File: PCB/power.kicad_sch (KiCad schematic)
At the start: 1 part, among them U2 LTC3370

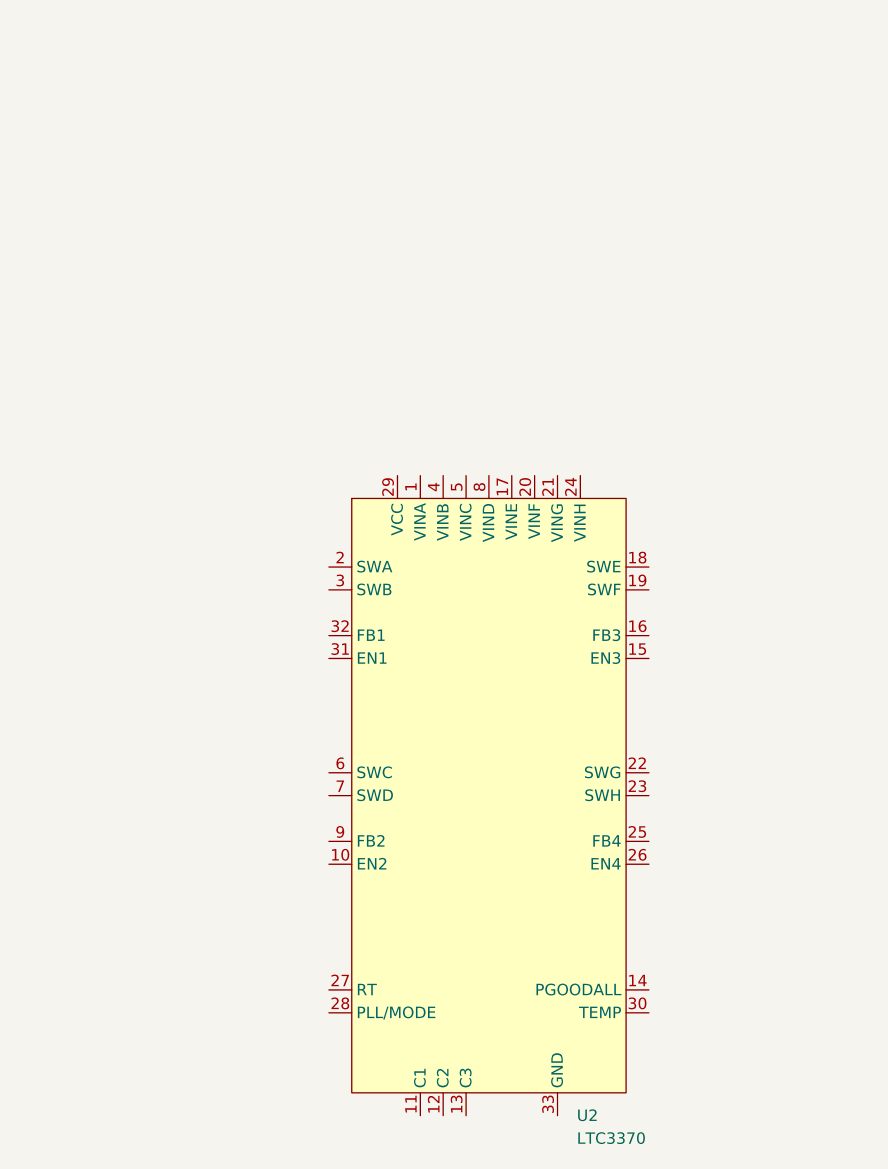
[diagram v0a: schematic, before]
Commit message: basic decoupling and config for quad buck
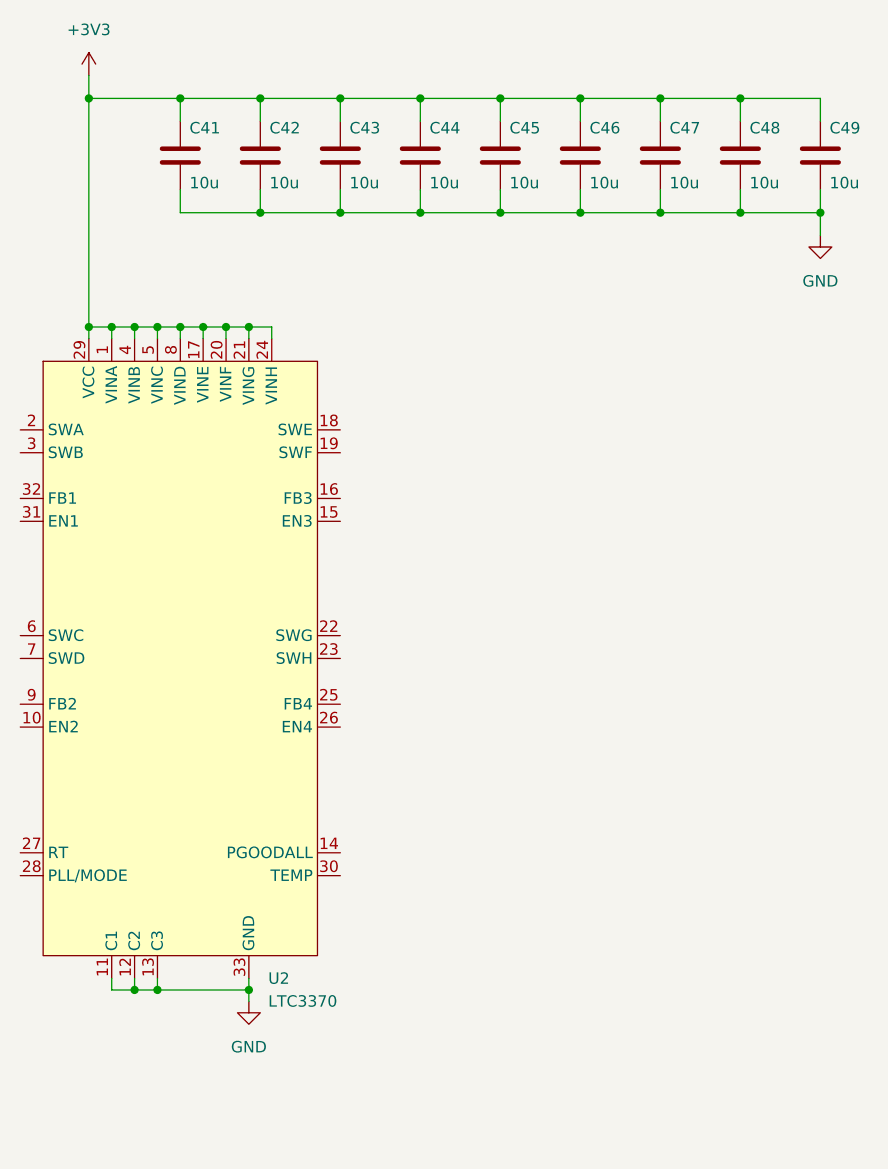
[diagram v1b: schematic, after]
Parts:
- added C41, C42, C43, C44, C45, C46, C47, C48, C49: 10u, symbol Device:C
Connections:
- net +3V3: now reaches U2.1 (VINA)
- net +3V3: now also U2.17 (VINE), U2.20 (VINF), U2.21 (VING), U2.24 (VINH), U2.29 (VCC), U2.4 (VINB), U2.5 (VINC), U2.8 (VIND), C41.1, C42.1, C43.1, C44.1, C45.1, C46.1, C47.1, C48.1, C49.1
- net GND: now reaches U2.11 (C1)
- net GND: now also U2.12 (C2), U2.13 (C3), U2.33 (GND), C41.2, C42.2, C43.2, C44.2, C45.2, C46.2, C47.2, C48.2, C49.2
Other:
- moved on the sheet: U2
